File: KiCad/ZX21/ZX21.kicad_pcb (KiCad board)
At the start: 2 copper layers, 142 x 100 mm, 128 parts, among them IC1 ULA 2C210E, IC101 555, IC102 74HCT00, IC2 AT28C256, IC3 Z80A, IC301 3V3 PSU, IC302 ESP32-WROOM, IC303 AZ1117-3.3, IC4 62256, IC501 YM2149, IC502 GAL16V8, IC801 AS6C4008Extra, J1 Jack-DC, J2 Conn_01x02, J203 Conn_01x03, J204 Conn_01x03, J301 Conn_01x04, J401 DB9_Male, J501 Conn_01x06, J502 Conn_01x08, J503 Conn_01x08, J504 Conn_01x07, J601 Conn_02x08_Odd_Even, J701 Conn_02x23_Row_Letter_First, J702 Conn_01x09, J703 Conn_01x09, X1 3.5MHz, X501 ECS-100AX-040

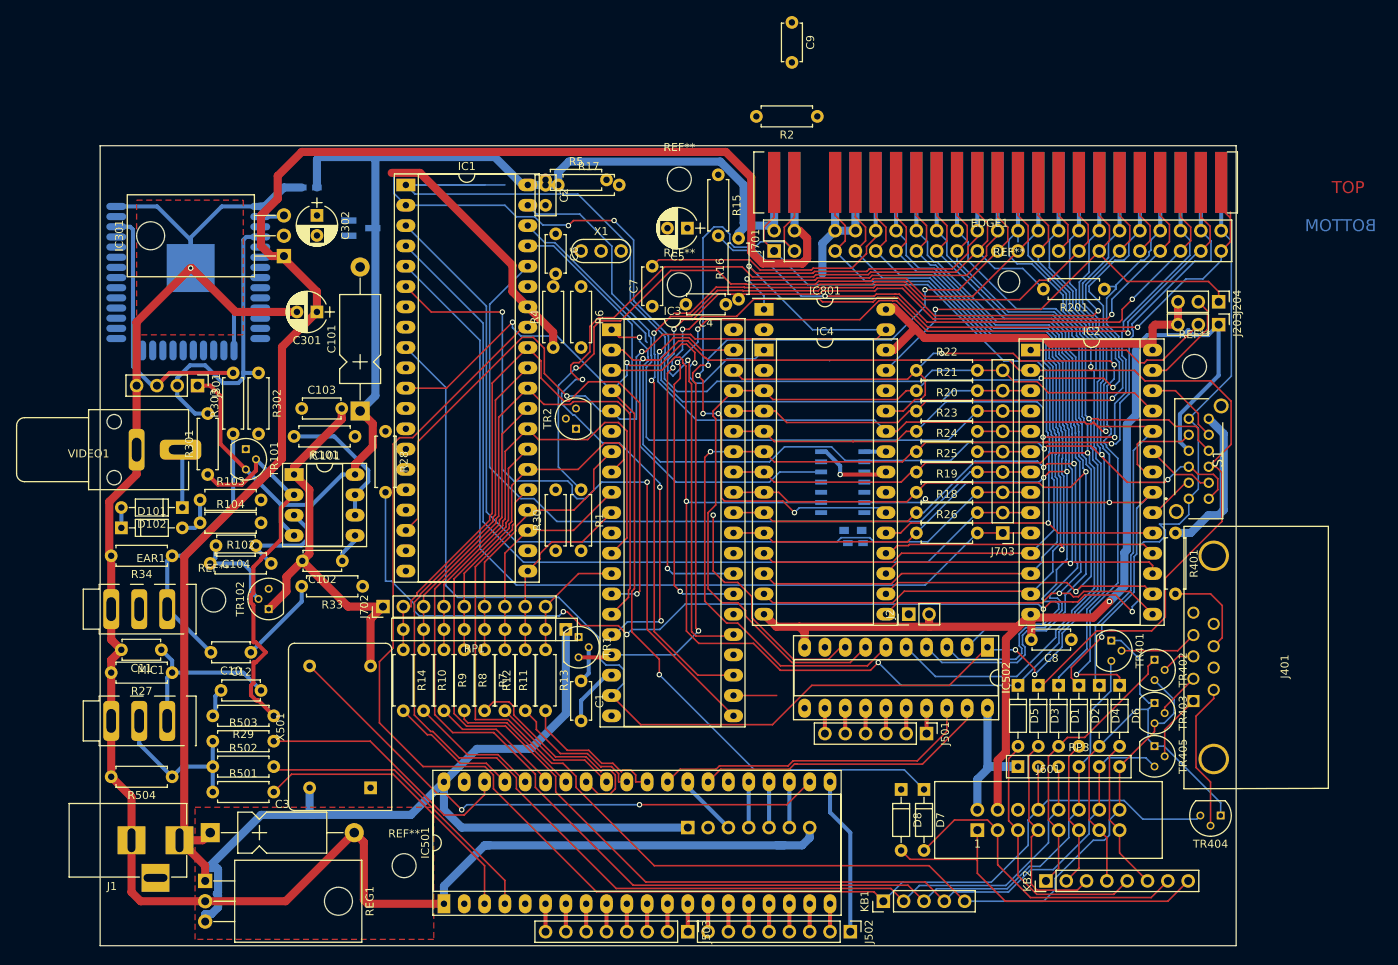
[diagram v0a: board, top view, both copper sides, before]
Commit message: Yup more routing
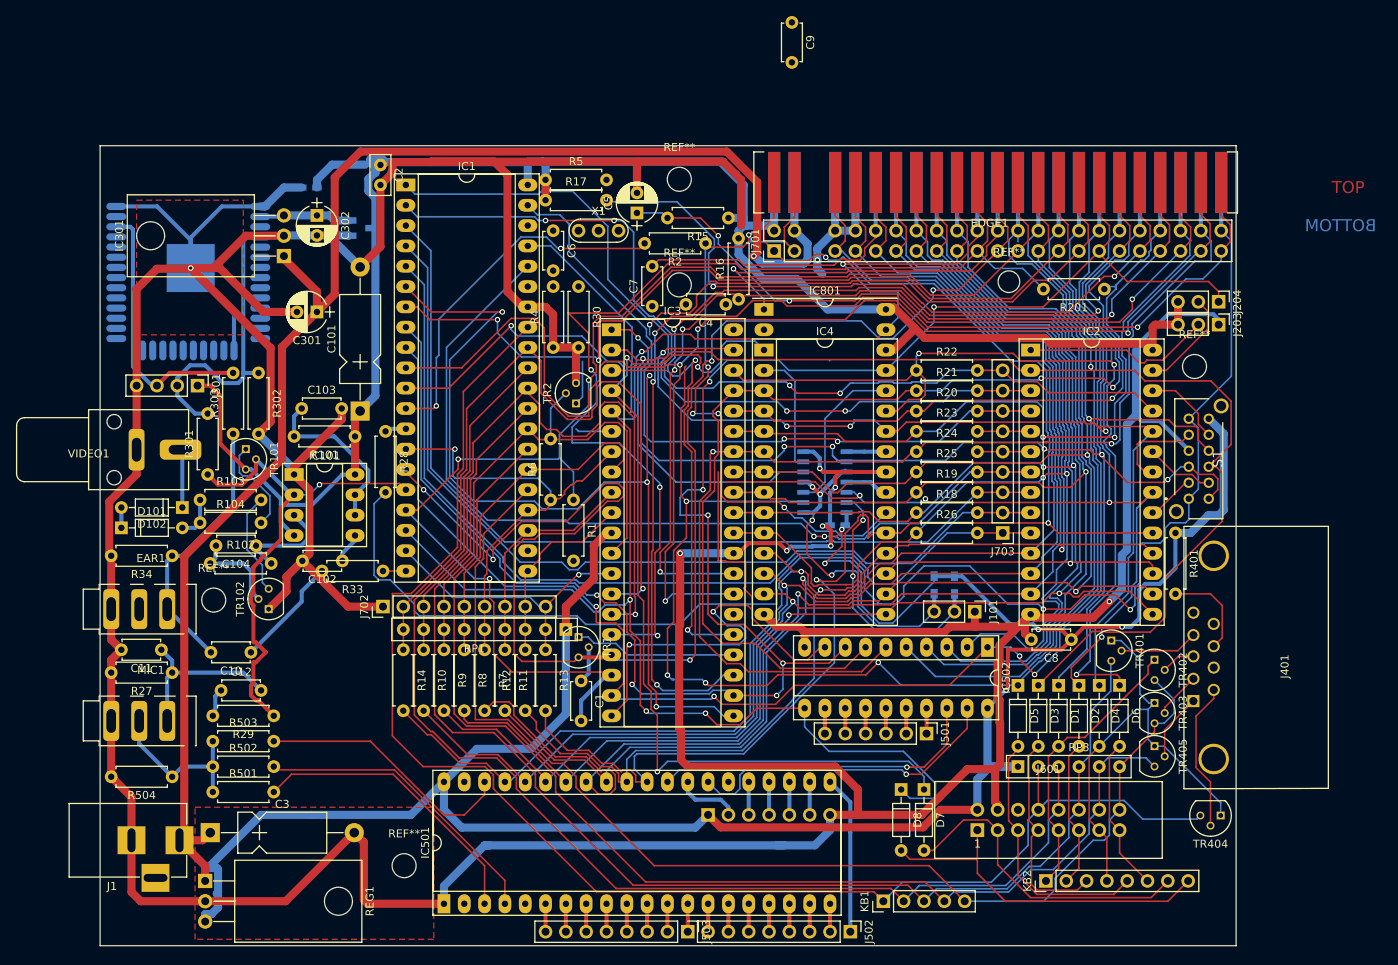
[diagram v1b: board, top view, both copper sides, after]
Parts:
- removed J2: Conn_01x02, Pin_Headers:Pin_Header_Straight_1x02_Pitch2.54mm
- removed X501: ECS-100AX-040, Oscillators:Oscillator_DIP-14
- added J101: Conn_01x03, Pin_Headers:Pin_Header_Straight_1x03_Pitch2.54mm, F.Cu at (140.3, 95.2)
- added R106: 10K, Resistors_SMD:R_0603_HandSoldering, B.Cu at (137.8, 91.9)
- R105: value 4K7 -> 10K
- moved R30 33.1 mm to (90.8, 54.6), turned to 270 degrees
- moved R6 26.9 mm to (87.3, 81.3), turned to 90 degrees
- moved R2 21.1 mm to (106.7, 49.2)
- moved C2 20.8 mm to (66.0, 39.4)
- moved R105 12.2 mm to (135.3, 91.9), turned to 90 degrees
- moved C5 6.59 mm to (98.1, 45.4), turned to 90 degrees
- moved R15 5.54 mm to (109.5, 46.0), turned to 180 degrees
- moved R33 3.18 mm to (66.4, 90.2)
- moved TR2 3.17 mm to (90.5, 69.2)
- moved C105 3.14 mm to (123.2, 84.5)
- moved J504 3.00 mm to (107.0, 120.7)
- moved X1 2.56 mm to (90.8, 47.6)
- moved R17 2.48 mm to (86.7, 43.8)
- moved IC102 2.22 mm to (121.6, 79.1)
- moved R1 1.59 mm to (90.2, 81.3)
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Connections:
- IC102 pad 13: Net-(IC102-Pad1) -> Net-(IC102-Pad13)
- J504 pad 2: Net-(J504-Pad2) -> Net-(IC501-Pad28)
- J504 pad 3: Net-(IC501-Pad28) -> Net-(IC501-Pad25)
- J504 pad 4: Net-(IC501-Pad25) -> Net-(IC501-Pad24)
- J504 pad 5: Net-(IC501-Pad24) -> Net-(IC501-Pad23)
- J504 pad 6: Net-(IC501-Pad23) -> Net-(IC501-Pad22)
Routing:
- net GND: track 508.3 -> 748.6 mm, vias 3 -> 9
- net +5V: track 356.8 -> 526.5 mm, vias 0 -> 5
- net IORQ: track 9.53 -> 176.7 mm, vias 0 -> 4
- net WR: track 97.4 -> 227.6 mm, vias 2 -> 8
- net WAIT: track 9.62 -> 110.8 mm, vias 0 -> 2
- net NMI: track 104.6 -> 185.5 mm, vias 4 -> 6
- net Net-(IC501-Pad22): track 71.4 -> 4.13 mm, vias 2 -> 0
- net D7': track 121.9 -> 186.4 mm, vias 1 -> 3
- net HALT: track 101.2 -> 164.3 mm, vias 1 -> 3
- net D0': track 119.2 -> 179.3 mm, vias 0 -> 1
- net D5': track 113.7 -> 170.9 mm, vias 1 -> 2
- net MI: track 122.1 -> 177.9 mm
- net A15: track 149.8 -> 205.4 mm, vias 3 -> 5
- net D4': track 126.0 -> 181.0 mm, vias 1 -> 2
- net D3': track 117.5 -> 171.7 mm, vias 1 -> 2
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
